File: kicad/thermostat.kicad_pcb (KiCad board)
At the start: 2 copper layers, 100.5 x 79.5 mm, 80 parts, among them IC1 LM2596S-5, J1 Conn_01x05, J2 Conn_02x02_Top_Bottom, J3 Conn_01x04, J4 Conn_01x04, J6 Screw_Terminal_01x05, SW1 Button, SW2 Button, SW3 Button, SW4 Button, T1 SIR434DN, T2 SIR434DN, U1 MCP23017_ML, U11 LTC4041, U21 BME280

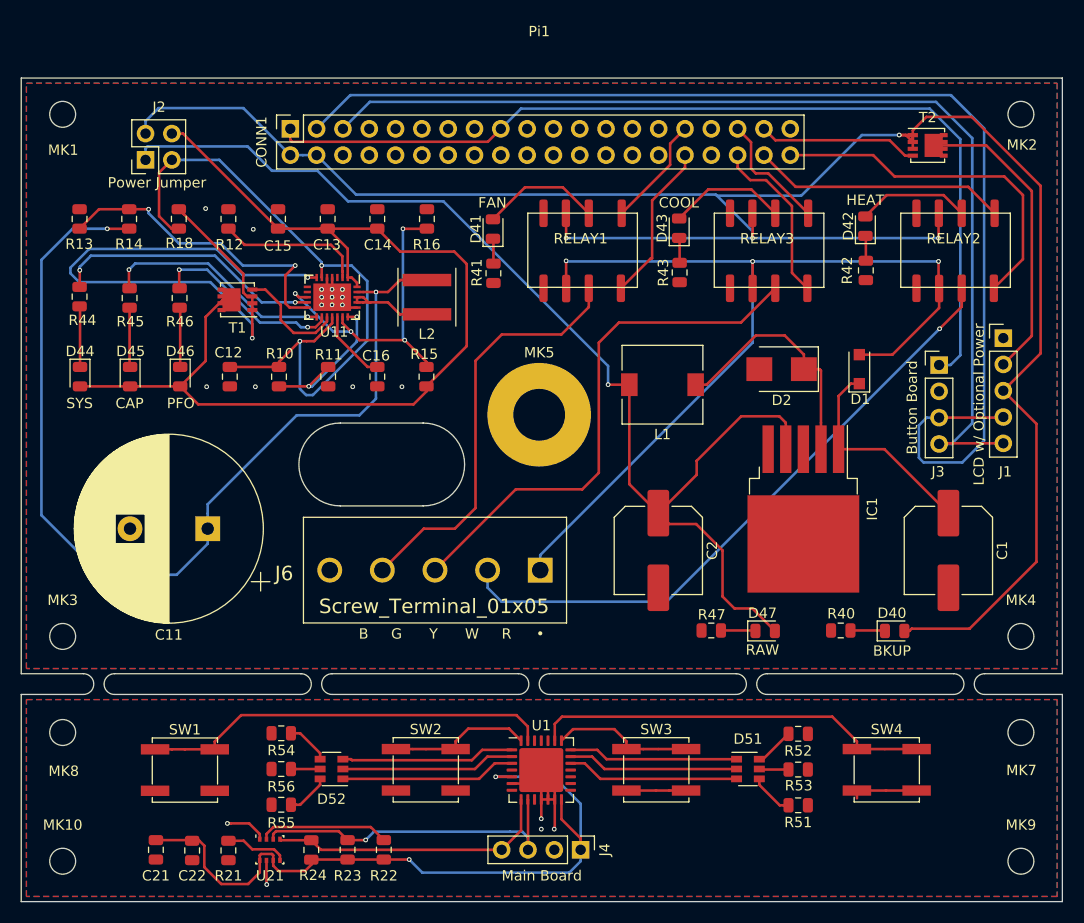
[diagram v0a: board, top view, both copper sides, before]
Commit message: routed board
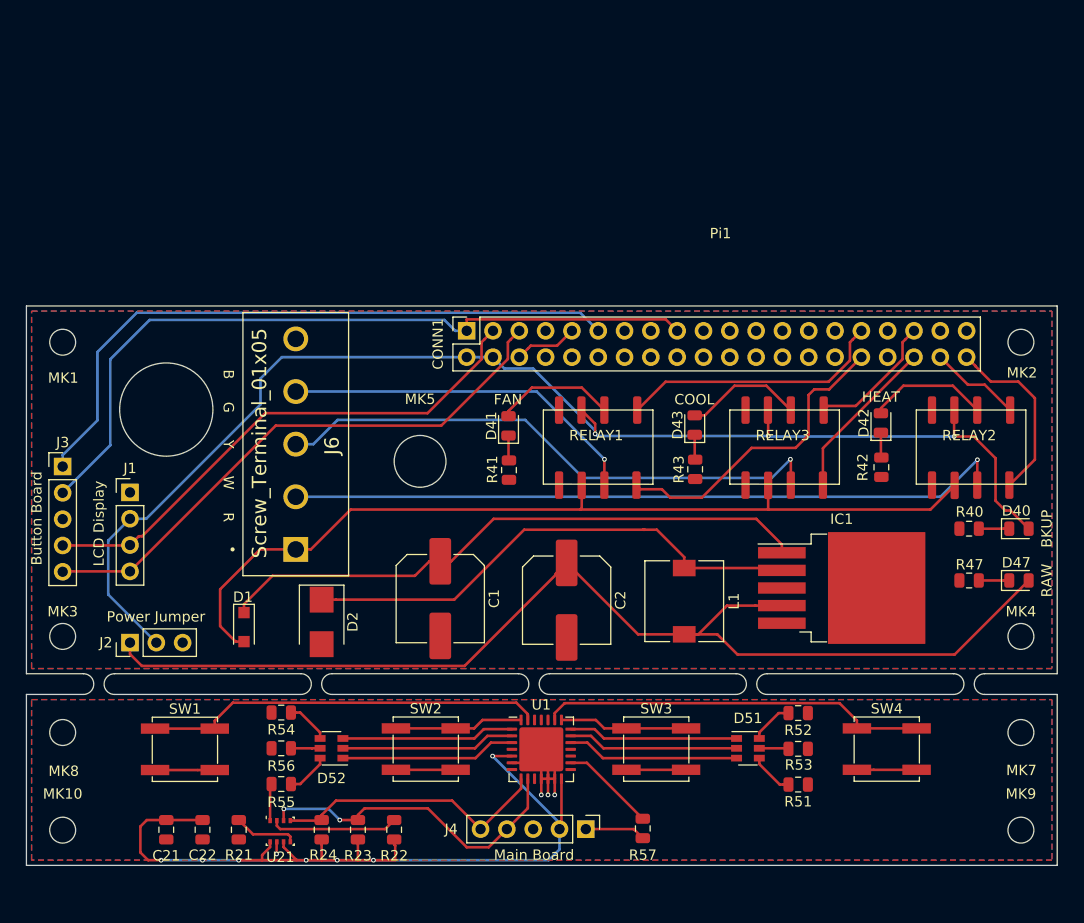
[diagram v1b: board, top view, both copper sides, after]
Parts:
- removed C11: 25F, Capacitor_THT:CP_Radial_D18.0mm_P7.50mm
- removed C12: 2.2uF, Capacitor_SMD:C_0805_2012Metric
- removed C13, C14: 100uF, Capacitor_SMD:C_0805_2012Metric
- removed C15, C16: 100nF, Capacitor_SMD:C_0805_2012Metric
- removed D44, D45, D46: Green, LED_SMD:LED_0805_2012Metric
- removed L2: 2.2uH, Inductor_SMD:L_Coilcraft_XAL5030
- removed R10: 120k, Resistor_SMD:R_0805_2012Metric
- removed R11: 39k, Resistor_SMD:R_0805_2012Metric
- removed R12, R44, R45, R46: 1k, Resistor_SMD:R_0805_2012Metric
- removed R13: 294k, Resistor_SMD:R_0805_2012Metric
- removed R14: 698k, Resistor_SMD:R_0805_2012Metric
- removed R15: 1050k, Resistor_SMD:R_0805_2012Metric
- removed R16: 200k, Resistor_SMD:R_0805_2012Metric
- removed R18: 10m, Resistor_SMD:R_0805_2012Metric
- removed T1, T2: SIR434DN, Package_SO:Vishay_PowerPAK_1212-8_Single
- removed U11: LTC4041, project_footprints:ltc4041
- added R57: 10k, Resistor_SMD:R_0805_2012Metric, F.Cu at (210.0, 189.9)
- J1: value Conn_01x05 -> Conn_01x04; footprint Connector_PinHeader_2.54mm:PinHeader_1x05_P2.54mm_Vertical -> Connector_PinHeader_2.54mm:PinHeader_1x04_P2.54mm_Vertical
- J2: value Conn_02x02_Top_Bottom -> Conn_01x03; footprint Connector_PinHeader_2.54mm:PinHeader_2x02_P2.54mm_Vertical -> Connector_PinHeader_2.54mm:PinHeader_1x03_P2.54mm_Vertical
- J3, J4: value Conn_01x04 -> Conn_01x05; footprint Connector_PinHeader_2.54mm:PinHeader_1x04_P2.54mm_Vertical -> Connector_PinHeader_2.54mm:PinHeader_1x05_P2.54mm_Vertical
- MK5: footprint MountingHole:MountingHole_5mm_Pad -> MountingHole:MountingHole_5mm
- moved J1 85.6 mm to (160.5, 157.5)
- moved J3 85.2 mm to (154.0, 155.0)
- moved D1 64.4 mm to (171.5, 170.5), turned to 270 degrees
- moved D2 50.7 mm to (179.0, 170.0), turned to 270 degrees
- moved C1 49.3 mm to (190.4, 167.8)
- moved J2 46.6 mm to (160.5, 172.0)
- moved Pi1 26.2 mm to (217.5, 131.5)
- moved CONN1 25.9 mm to (193.0, 141.9)
- moved R47 25.4 mm to (241.5, 166.0)
- moved D47 25.0 mm to (246.3, 166.0)
- moved J6 23.7 mm to (176.5, 163.0), turned to 90 degrees
- moved MK1 22.0 mm to (154.0, 143.0)
- moved MK2 22.0 mm to (246.5, 143.0)
- moved L1 21.0 mm to (214.0, 168.0), turned to 270 degrees
- moved D41 19.1 mm to (197.0, 151.1)
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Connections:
- CONN1 pad 11: (no net) -> /GPIO17(GEN0)
- CONN1 pad 37: /GPIO26 -> (no net)
- J1 pad 2: Net-(J1-Pad2) -> /PWR_5V
- J1 pad 3: /PWR_5V -> /GPIO2(SDA1)
- J1 pad 4: /GPIO2(SDA1) -> /GPIO3(SCL1)
- J2 pad 3: /PWR_CAP_IN -> GND
- J3 pad 1: /PWR_3.3V -> /GPIO17(GEN0)
- J3 pad 2: GND -> /PWR_3.3V
- J3 pad 3: /GPIO2(SDA1) -> GND
- J3 pad 4: /GPIO3(SCL1) -> /GPIO2(SDA1)
- J4 pad 1: /BTNS_PWR_3V3 -> /BTNS_INT
- J4 pad 2: /BTNS_GND -> /BTNS_PWR_3V3
- J4 pad 3: /BTNS_SDA -> /BTNS_GND
- J4 pad 4: /BTNS_SCL -> /BTNS_SDA
- U1 pad 16: (no net) -> Net-(R57-Pad2)
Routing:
- net /PWR_CAP_OUT: track 100.2 -> 0.00 mm
- net Net-(C11-Pad1): track 95.8 -> 0.00 mm, vias 2 -> 0
- net /PWR_5V: track 204.7 -> 126.8 mm, vias 4 -> 3
- net /PWR_CAP_IN: track 65.2 -> 0.00 mm, vias 2 -> 0
- net /GPIO2(SDA1): track 116.2 -> 51.1 mm
- net /GPIO17(GEN0): track 0.00 -> 63.1 mm
- net Net-(R18-Pad1): track 62.8 -> 0.00 mm, vias 2 -> 0
- net /GPIO3(SCL1): track 101.0 -> 54.7 mm
- net Net-(C1-Pad1): track 20.8 -> 58.0 mm
- net Net-(R15-Pad1): track 32.1 -> 0.00 mm, vias 4 -> 0
- net Net-(R13-Pad1): track 30.4 -> 0.00 mm, vias 2 -> 0
- net Net-(J1-Pad2): track 29.2 -> 0.00 mm
- net /SYSGD: track 26.2 -> 0.00 mm, vias 2 -> 0
- net Net-(D2-Pad1): track 23.9 -> 49.6 mm
- net /BTNS_PWR_3V3: track 71.2 -> 94.0 mm, vias 2 -> 7
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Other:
- board size 100.5 x 79.5 mm -> 99.5 x 54 mm
- board text added: "LCD Display"
- board text removed: "CAP"
- board text removed: "LCD w/ Optional Power"
- board text removed: "PFO"
- board text removed: "SYS"
